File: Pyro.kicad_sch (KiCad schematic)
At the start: 36 parts, among them J12 Conn_01x02_Male, Q2 BUK9M11-40EX, U10 SiC437BED-T1-GE3, U11 TPS259621DDAT, U9 859-LTV-247

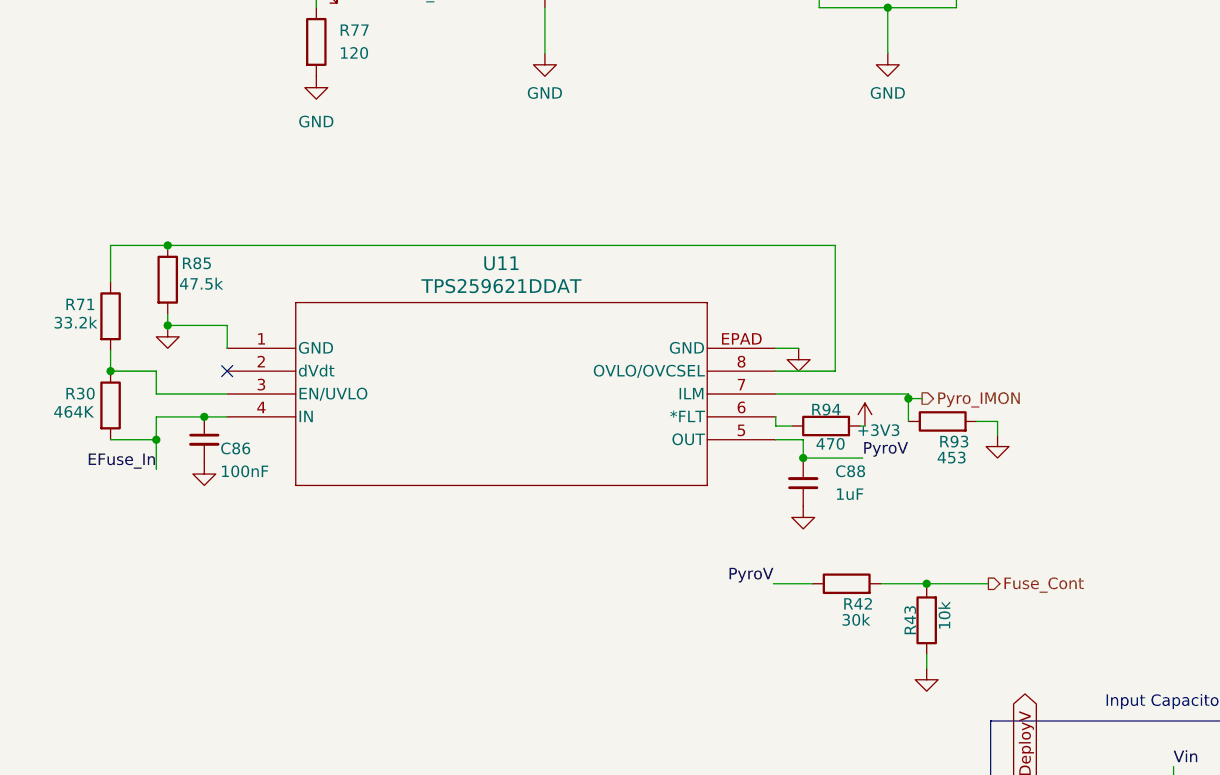
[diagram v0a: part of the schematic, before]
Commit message: more changes
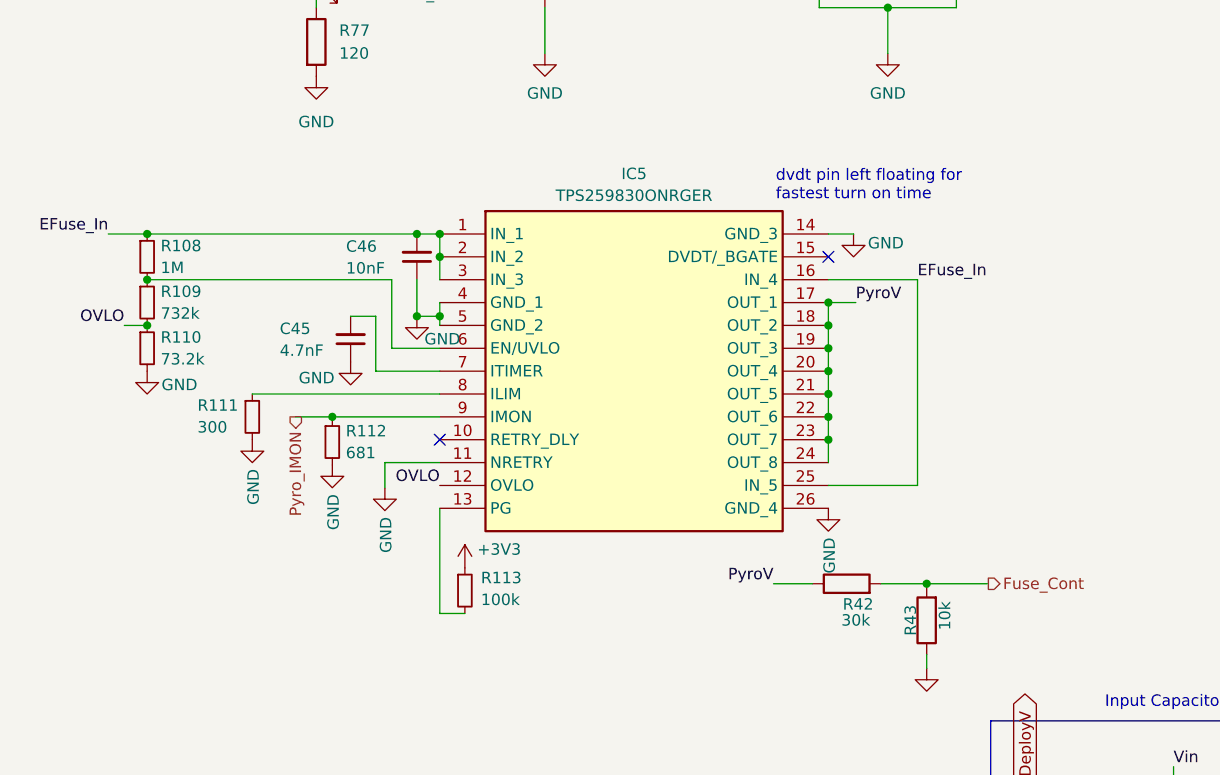
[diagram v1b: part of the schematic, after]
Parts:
- removed C86: 100nF, Capacitor_SMD:C_0402_1005Metric, symbol Device:C_Small
- removed C88: 1uF, Capacitor_SMD:C_0603_1608Metric, symbol Device:C_Small
- removed R30: 464K, Resistor_SMD:R_0402_1005Metric, symbol Device:R
- removed R71: 33.2k, Resistor_SMD:R_0402_1005Metric, symbol Device:R
- removed R85: 47.5k, Resistor_SMD:R_0402_1005Metric, symbol Device:R
- removed R93: 453, Resistor_SMD:R_0402_1005Metric, symbol Device:R
- removed R94: 470, Resistor_SMD:R_0402_1005Metric, symbol Device:R
- removed U11: TPS259621DDAT, EFuse:SO-PP-DDA-8_TEX, symbol EFuse:TPS259621DDAT
- added C45: 4.7nF, Capacitor_SMD:C_0402_1005Metric, symbol Device:C_Small
- added C46: 10nF, Capacitor_SMD:C_0402_1005Metric, symbol Device:C_Small
- added IC5: TPS259830ONRGER, iclr:TPS259830ONRGER, symbol iclr:TPS259830ONRGER
- added R108: 1M, Capacitor_SMD:C_0402_1005Metric, symbol Device:R_Small
- added R109: 732k, Capacitor_SMD:C_0402_1005Metric, symbol Device:R_Small
- added R110: 73.2k, Capacitor_SMD:C_0402_1005Metric, symbol Device:R_Small
- added R111: 300, Capacitor_SMD:C_0402_1005Metric, symbol Device:R_Small
- added R112: 681, Capacitor_SMD:C_0402_1005Metric, symbol Device:R_Small
- added R113: 100k, Capacitor_SMD:C_0402_1005Metric, symbol Device:R_Small
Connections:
- net +3V3: now also R113.1
- net EFuse_In: now also C46.2, IC5.1 (IN_1), IC5.16 (IN_4), IC5.2 (IN_2), IC5.25 (IN_5), IC5.3 (IN_3), R108.1
- net GND: now also C45.1, C46.1, IC5.11 (NRETRY), IC5.14 (GND_3), IC5.26 (GND_4), IC5.4 (GND_1), IC5.5 (GND_2), R110.2, R111.2, R112.2
- net PyroV: now also IC5.17 (OUT_1), IC5.18 (OUT_2), IC5.19 (OUT_3), IC5.20 (OUT_4), IC5.21 (OUT_5), IC5.22 (OUT_6), IC5.23 (OUT_7), IC5.24 (OUT_8)
- net Pyro_IMON: now also IC5.9 (IMON), R112.1
- new net: IC5.8 (ILIM), R111.1
- new net: C45.2, IC5.7 (ITIMER)
- new net: IC5.13 (PG), R113.2
- new net: IC5.6 (EN/UVLO), R108.2, R109.1
- new net OVLO: IC5.12 (OVLO), R109.2, R110.1
- no-connect marks 4 -> 5
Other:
- note added: "dvdt pin left floating for fastest turn on time"
